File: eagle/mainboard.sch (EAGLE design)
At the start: 55 parts, among them IC1 74HCT151D, IC2 74HCT151D, IC3 74HCT151D, IC4 74HCT151D, IC5 74HCT151D, IC6 74HCT151D, IC7 74HC590D, IC8 74HC02D, J1 632723100011_USBC_3.1, J2 632723100011_USBC_3.1, J3 632723100011_USBC_3.1, J4 632723100011_USBC_3.1, J5 632723100011_USBC_3.1, J7 L77HDE15SD1CH4RHNVGA

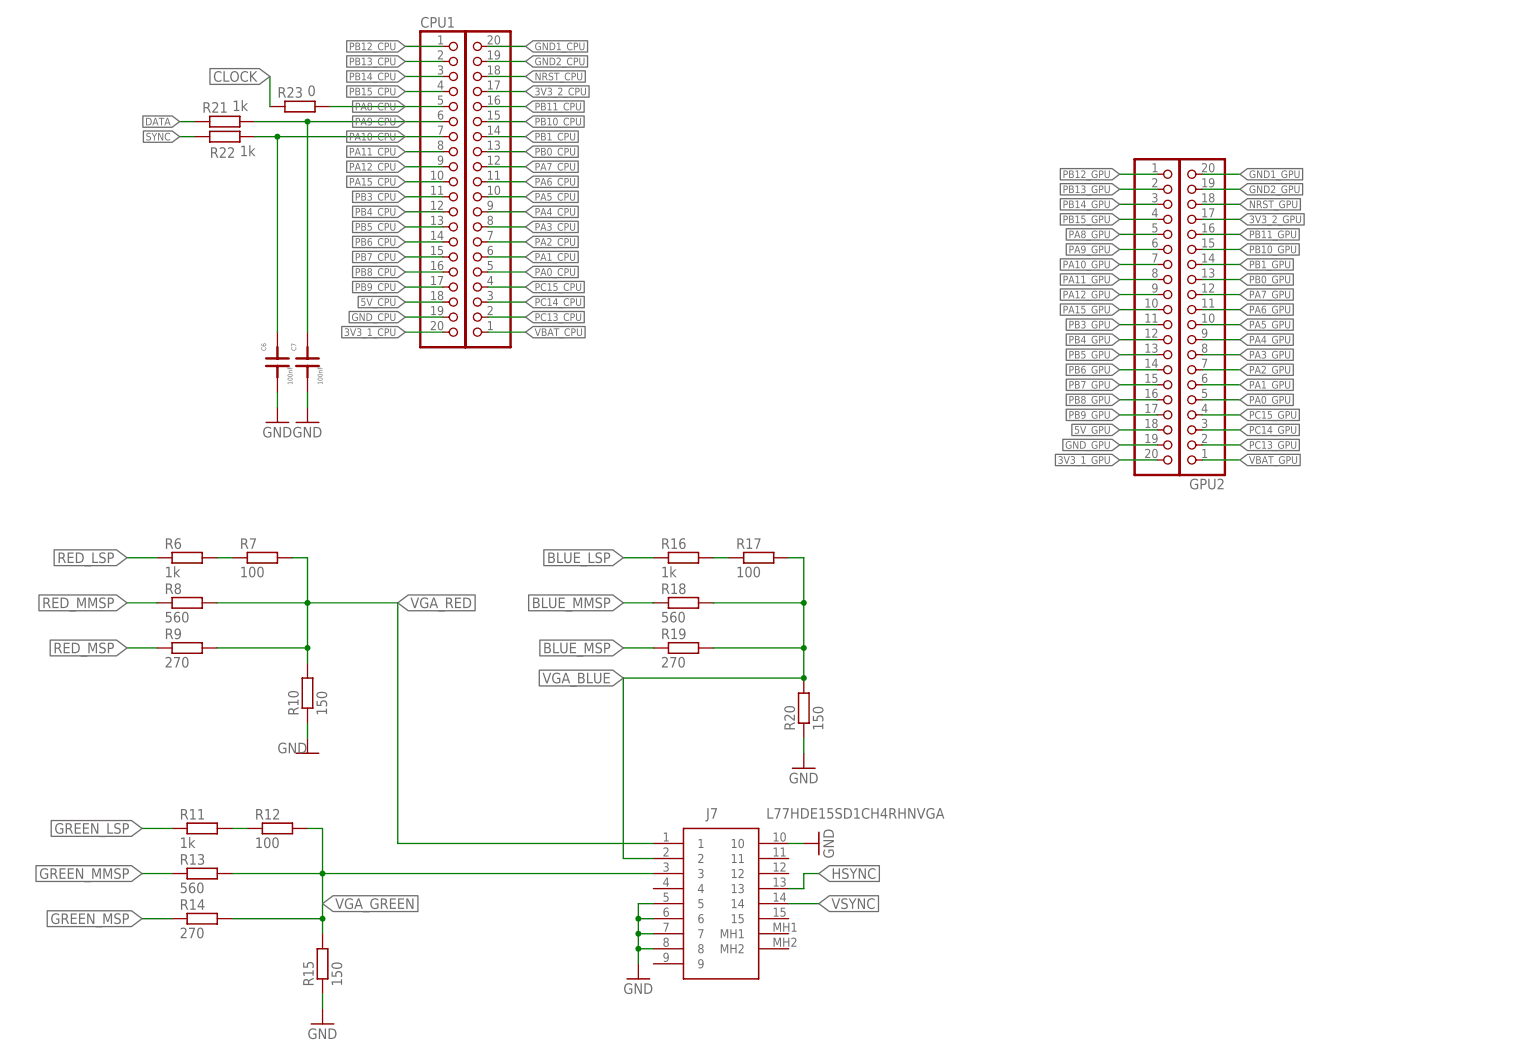
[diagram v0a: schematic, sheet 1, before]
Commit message: fixed schematic
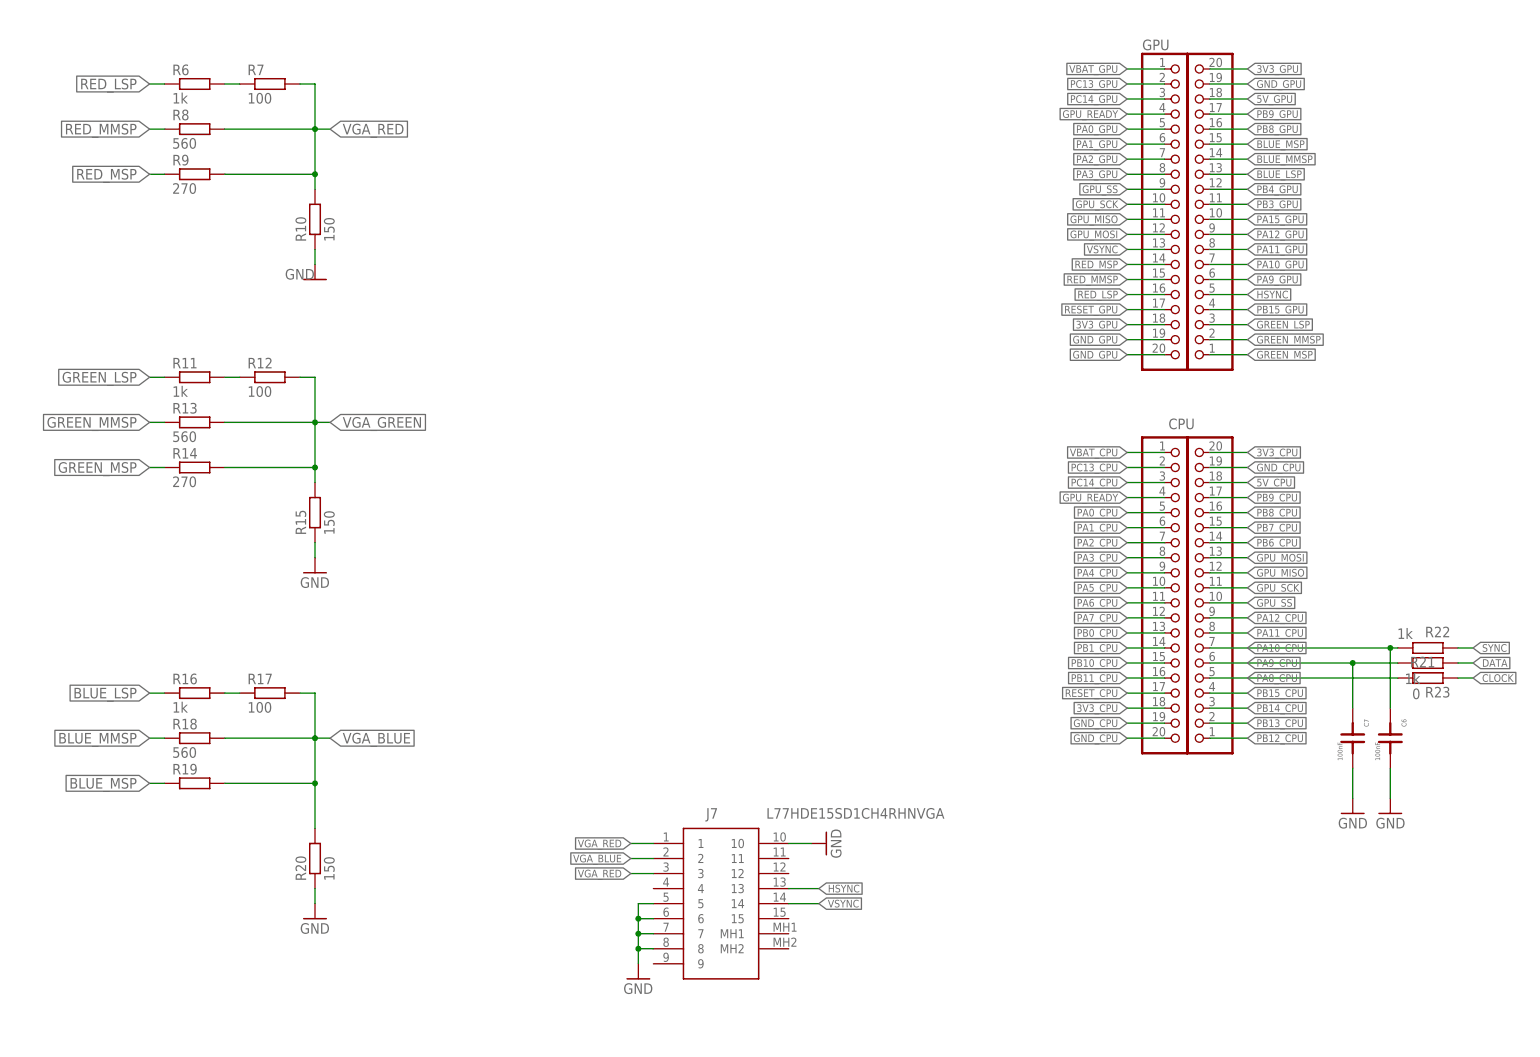
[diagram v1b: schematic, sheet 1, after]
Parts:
- removed CPU1, GPU2: (no value), pinhead:PINHD-1X20
- added CPU, GPU: (no value), pinhead:PINHD-1X20
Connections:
- net 3V3_2_CPU renamed RESET_CPU
- removed net 3V3_1_CPU: CPU1.20
- removed net 3V3_1_GPU: GPU1.20
- removed net 3V3_2_GPU: GPU2.17
- removed net GND1_CPU: CPU2.20
- removed net GND1_GPU: GPU2.20
- removed net GND2_CPU: CPU2.19
- removed net GND2_GPU: GPU2.19
- removed net NRST_CPU: CPU2.18
- removed net NRST_GPU: GPU2.18
- removed net PA15_CPU: CPU1.10
- removed net PA4_GPU: GPU2.9
- removed net PA5_GPU: GPU2.10
- removed net PA6_GPU: GPU2.11
- removed net PA7_GPU: GPU2.12
- removed net PA8_GPU: GPU1.5
- removed net PB0_GPU: GPU2.13
- removed net PB10_GPU: GPU2.15
- removed net PB11_GPU: GPU2.16
- removed net PB12_GPU: GPU1.1
- removed net PB13_GPU: GPU1.2
- removed net PB14_GPU: GPU1.3
- removed net PB1_GPU: GPU2.14
- removed net PB3_CPU: CPU1.11
- removed net PB4_CPU: CPU1.12
- removed net PB5_CPU: CPU1.13
- removed net PB5_GPU: GPU1.13
- removed net PB6_GPU: GPU1.14
- removed net PB7_GPU: GPU1.15
- removed net PC15_CPU: CPU2.4
- removed net PC15_GPU: GPU2.4
- new net 3V3_CPU: CPU.20, CPU2.18
- new net 3V3_GPU: GPU.18, GPU1.20
- new net GPU_MISO: CPU.12, GPU.11
- new net GPU_MOSI: CPU.13, GPU.12
- new net GPU_READY: CPU2.4, GPU.4
- new net GPU_SCK: CPU.11, GPU.10
- new net GPU_SS: CPU.10, GPU.9
- new net RESET_GPU: GPU.17
- net 5V_CPU: now also CPU.18; no longer CPU1.18
- net BLUE_LSP: now also GPU1.13
- net BLUE_MMSP: now also GPU1.14
- net BLUE_MSP: now also GPU1.15
- net GND_CPU: now also CPU.19, CPU2.19, CPU2.20; no longer CPU1.19
- net GND_GPU: now also GPU.19, GPU.20
- net GREEN_LSP: now also GPU1.3
- net GREEN_MMSP: now also GPU1.2
- net GREEN_MSP: now also GPU1.1
- net HSYNC: now also GPU1.5
- net PA0_GPU: now also GPU.5; no longer GPU2.5
- net PA10_CPU: now also CPU.7; no longer CPU1.7
- net PA11_CPU: now also CPU.8; no longer CPU1.8
- net PA12_CPU: now also CPU.9; no longer CPU1.9
- net PA1_GPU: now also GPU.6; no longer GPU2.6
- net PA2_GPU: now also GPU.7; no longer GPU2.7
- net PA3_GPU: now also GPU.8; no longer GPU2.8
- net PA8_CPU: now also CPU.5; no longer CPU1.5
- net PA9_CPU: now also CPU.6; no longer CPU1.6
- net PB12_CPU: now also CPU.1; no longer CPU1.1
- net PB13_CPU: now also CPU.2; no longer CPU1.2
- net PB14_CPU: now also CPU.3; no longer CPU1.3
- net PB15_CPU: now also CPU.4; no longer CPU1.4
- net PB6_CPU: now also CPU.14; no longer CPU1.14
- net PB7_CPU: now also CPU.15; no longer CPU1.15
- net PB8_CPU: now also CPU.16; no longer CPU1.16
- net PB9_CPU: now also CPU.17; no longer CPU1.17
- net PC13_GPU: now also GPU.2; no longer GPU2.2
- net PC14_GPU: now also GPU.3; no longer GPU2.3
- net RED_LSP: now also GPU.16
- net RED_MMSP: now also GPU.15
- net RED_MSP: now also GPU.14
- net VBAT_GPU: now also GPU.1; no longer GPU2.1
- net VGA_GREEN: no longer J7.3
- net VGA_RED: now also J7.3
- net VSYNC: now also GPU.13
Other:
- moved on the sheet: C6, C7, R10, R11, R12, R13, R14, R15, R16, R17, R18, R19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
